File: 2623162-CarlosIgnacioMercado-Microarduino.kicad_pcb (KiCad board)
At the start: 2 copper layers, 14 parts, among them J1 USB_A_UCC, J2 Header, U1 ATtiny85-20S

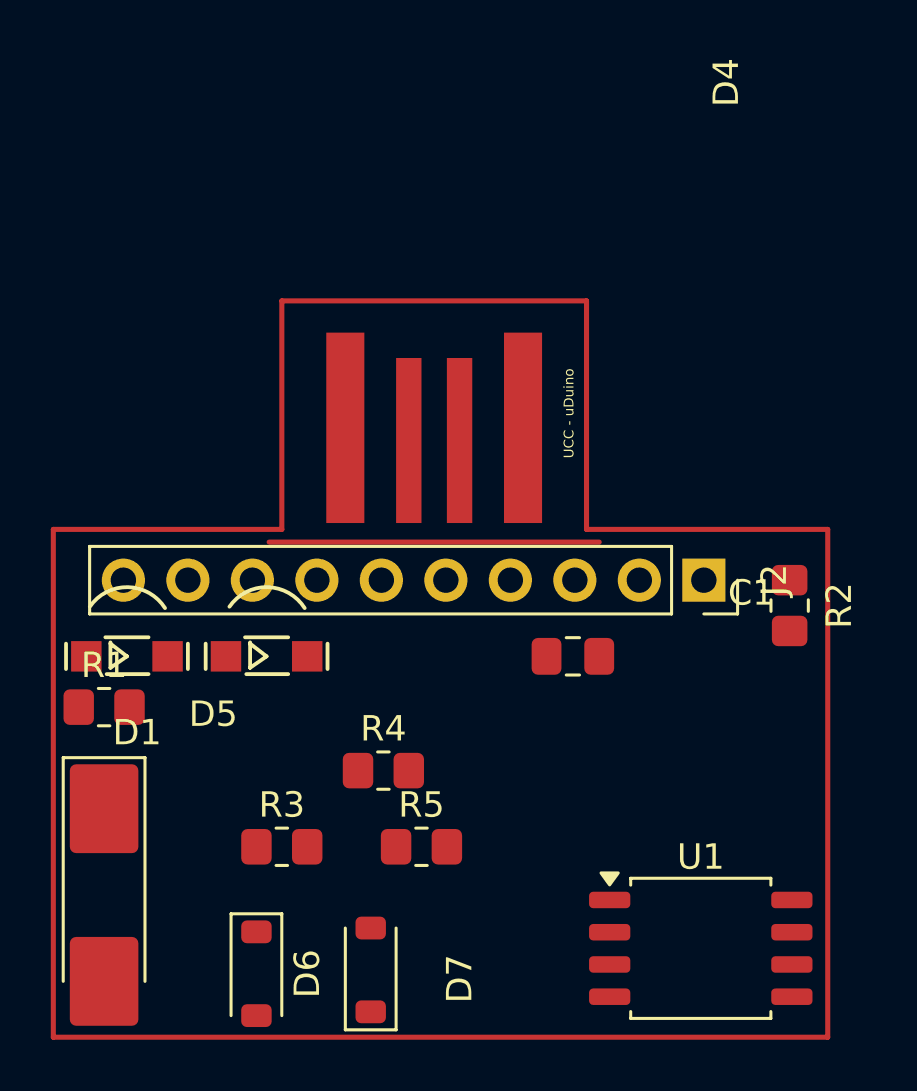
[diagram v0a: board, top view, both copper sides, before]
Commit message: cambios en el proyecto
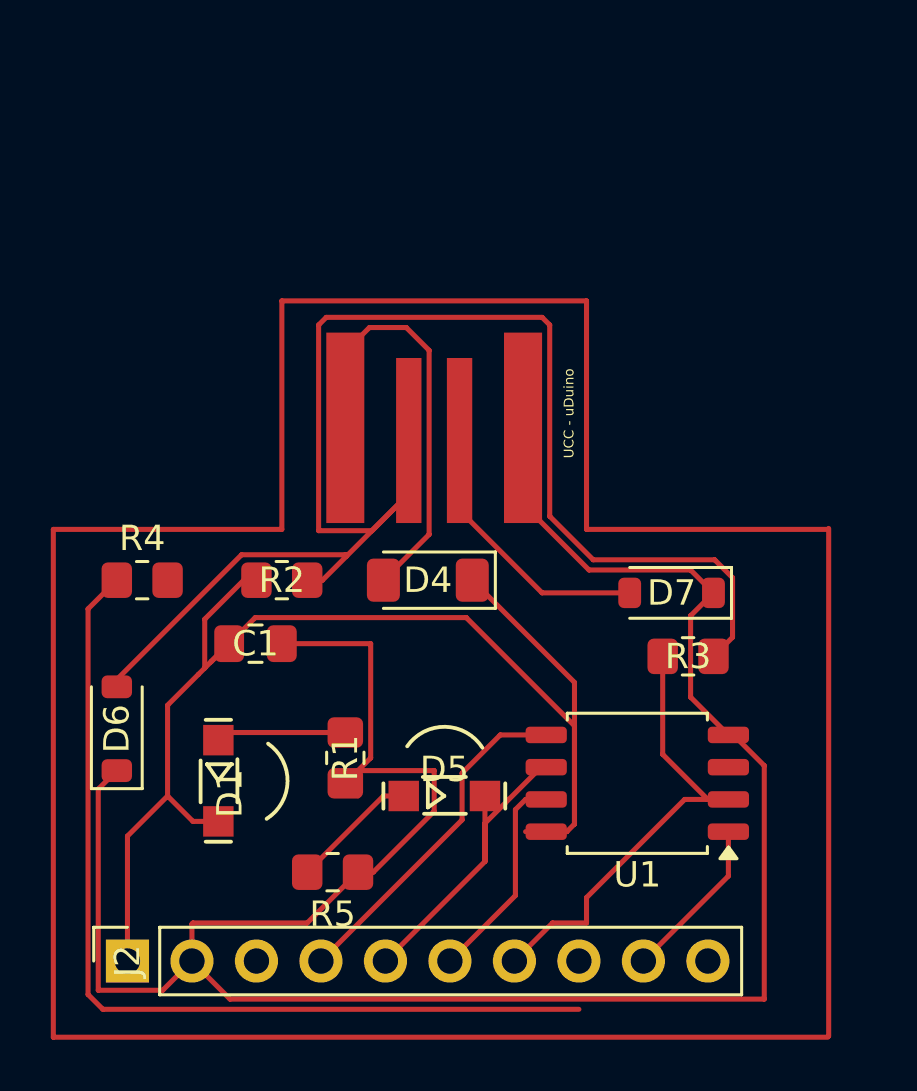
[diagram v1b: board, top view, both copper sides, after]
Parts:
- D4: footprint Diode_SMD:D_MELF_Handsoldering -> Diode_SMD:D_MiniMELF
- moved J2 27.2 mm to (138.4, 114.5), turned to 90 degrees
- moved R2 20.0 mm to (144.5, 99.5), turned to 0 degrees
- moved D7 19.0 mm to (159.8, 100.0), turned to 180 degrees
- moved D4 17.8 mm to (150.2, 99.5), turned to 180 degrees
- moved R3 17.7 mm to (160.5, 102.5)
- moved C1 12.5 mm to (143.5, 102.0)
- moved R4 12.1 mm to (139.0, 99.5)
- moved D6 11.1 mm to (138.0, 105.3), turned to 90 degrees
- moved R1 9.71 mm to (147.0, 106.5), turned to -90 degrees
- moved D5 8.90 mm to (151.4, 107.5)
- moved U1 6.96 mm to (158.5, 107.5), turned to 180 degrees
- moved D1 6.84 mm to (142.4, 107.9), turned to -90 degrees
- moved R5 3.64 mm to (146.5, 111.0), turned to 180 degrees
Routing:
- net GND: track 0.00 -> 94.2 mm
- net Net-(D6-A): track 0.00 -> 59.7 mm
- net +5V: track 0.00 -> 55.2 mm
- net Net-(J2-Pin_8): track 0.00 -> 36.4 mm
- net Net-(J2-Pin_7): track 0.00 -> 18.8 mm
- net Net-(D4-A): track 0.00 -> 16.9 mm
- net Net-(J2-Pin_4): track 0.00 -> 13.6 mm
- net Net-(D5-A): track 0.00 -> 13.0 mm
- net Net-(D7-A): track 0.00 -> 10.8 mm
- net Net-(J2-Pin_6): track 0.00 -> 8.41 mm
- net Net-(J2-Pin_9): track 0.00 -> 6.48 mm
- net Net-(D1-K): track 0.00 -> 5.12 mm
- net Net-(D5-K): track 0.00 -> 5.04 mm
